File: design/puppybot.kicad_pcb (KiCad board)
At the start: 2 copper layers, 1 part

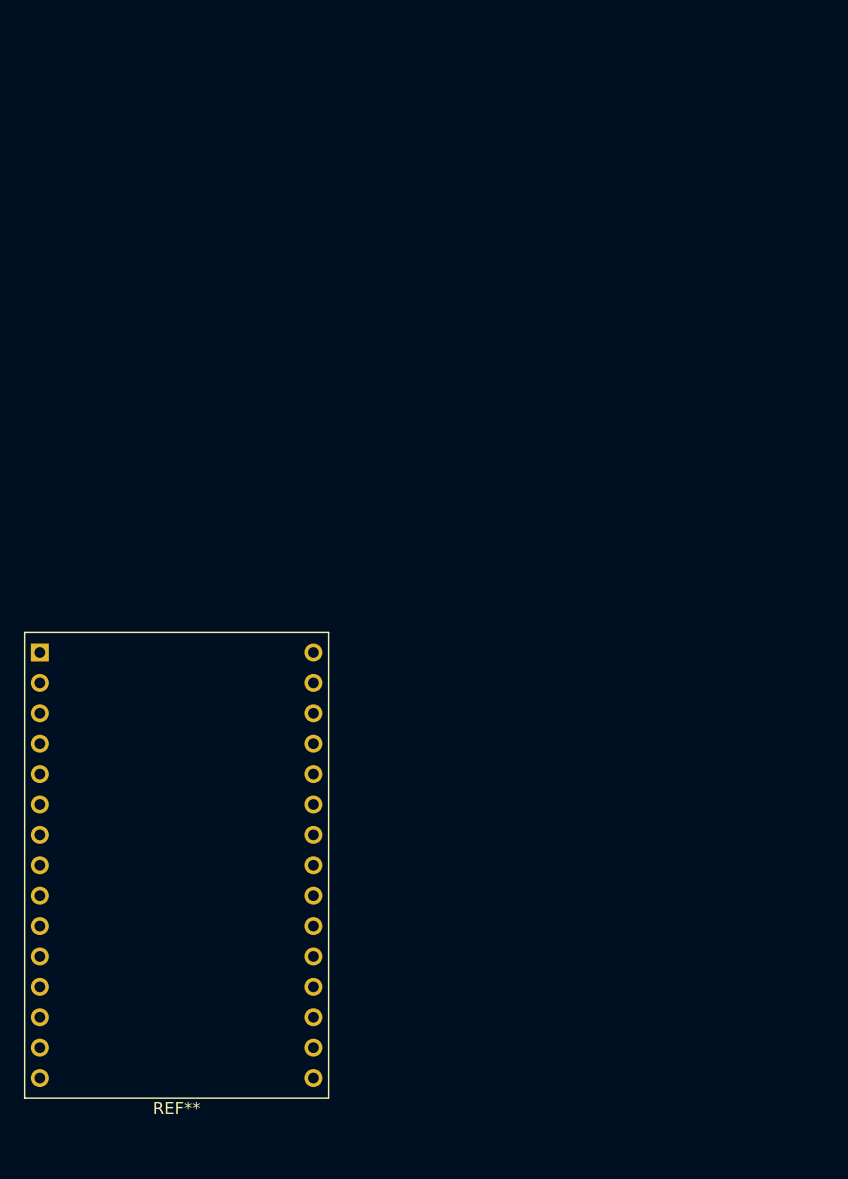
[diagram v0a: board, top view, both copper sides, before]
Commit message: update elecric design
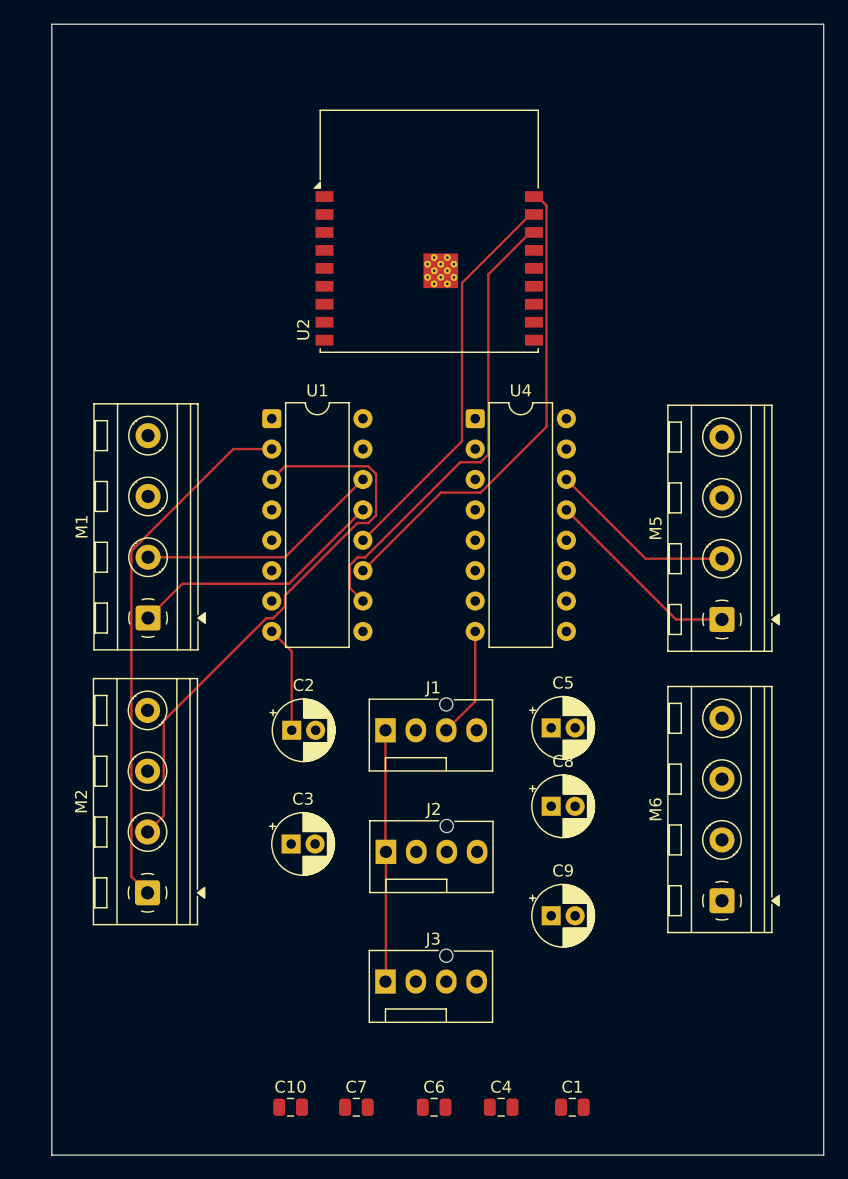
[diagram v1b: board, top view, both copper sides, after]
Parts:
- removed REF**: ESP32-C3-DevKitM-1, RF_Module:ESP32-C3-DevKitM-1
- added C1: C, Capacitor_SMD:C_0805_2012Metric, F.Cu at (159.0, 112.5)
- added C10: C, Capacitor_SMD:C_0805_2012Metric, F.Cu at (135.4, 112.5)
- added C2: C_Polarized, Capacitor_THT:CP_Radial_D5.0mm_P2.00mm, F.Cu at (135.5, 81.0)
- added C3: C_Polarized, Capacitor_THT:CP_Radial_D5.0mm_P2.00mm, F.Cu at (135.5, 90.5)
- added C4: C, Capacitor_SMD:C_0805_2012Metric, F.Cu at (153.1, 112.5)
- added C5: C_Polarized, Capacitor_THT:CP_Radial_D5.0mm_P2.00mm, F.Cu at (157.2, 80.8)
- added C6: C, Capacitor_SMD:C_0805_2012Metric, F.Cu at (147.4, 112.5)
- added C7: C, Capacitor_SMD:C_0805_2012Metric, F.Cu at (140.9, 112.5)
- added C8: C_Polarized, Capacitor_THT:CP_Radial_D5.0mm_P2.00mm, F.Cu at (157.2, 87.3)
- added C9: C_Polarized, Capacitor_THT:CP_Radial_D5.0mm_P2.00mm, F.Cu at (157.2, 96.5)
- added J1: XL4015, Connector:FanPinHeader_1x04_P2.54mm_Vertical, F.Cu at (143.4, 81.0)
- added J2: XL4015, Connector:FanPinHeader_1x04_P2.54mm_Vertical, F.Cu at (143.4, 91.2)
- added J3: XL4015, Connector:FanPinHeader_1x04_P2.54mm_Vertical, F.Cu at (143.4, 102.0)
- added M1: Motor_DC, TerminalBlock_RND:TerminalBlock_RND_205-00234_1x04_P5.08mm_Horizontal, F.Cu at (123.5, 71.6)
- added M2: Motor_DC, TerminalBlock_RND:TerminalBlock_RND_205-00234_1x04_P5.08mm_Horizontal, F.Cu at (123.5, 94.6)
- added M5: Motor_DC, TerminalBlock_RND:TerminalBlock_RND_205-00234_1x04_P5.08mm_Horizontal, F.Cu at (171.5, 71.7)
- added M6: Motor_DC, TerminalBlock_RND:TerminalBlock_RND_205-00234_1x04_P5.08mm_Horizontal, F.Cu at (171.5, 95.2)
- added U1: L298N, Package_DIP:DIP-16_W7.62mm, F.Cu at (133.9, 55.0)
- added U2: ESP32-C3-WROOM-02, RF_Module:ESP32-C3-WROOM-02, F.Cu at (147.0, 42.4)
- added U4: L298N, Package_DIP:DIP-16_W7.62mm, F.Cu at (150.9, 55.0)
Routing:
- net Net-(M2--): track 0.00 -> 48.1 mm
- net Net-(M2-+): track 0.00 -> 44.4 mm
- net Net-(U1-EnB): track 0.00 -> 40.2 mm
- net Net-(U1-IN3): track 0.00 -> 39.2 mm
- net Net-(U1-IN4): track 0.00 -> 33.3 mm
- net Net-(M1-+): track 0.00 -> 21.7 mm
- net Net-(J1-Pin_1): track 0.00 -> 21.0 mm
- net Net-(M1--): track 0.00 -> 20.6 mm
- net GND: track 0.00 -> 18.2 mm
- net Net-(M5-+): track 0.00 -> 16.8 mm
- net Net-(M5--): track 0.00 -> 15.7 mm
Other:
- board outline added: 64.5 x 94.5 mm
